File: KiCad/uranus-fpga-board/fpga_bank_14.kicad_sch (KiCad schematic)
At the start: 1 part, among them U12 XC7K325T-3FFG900E

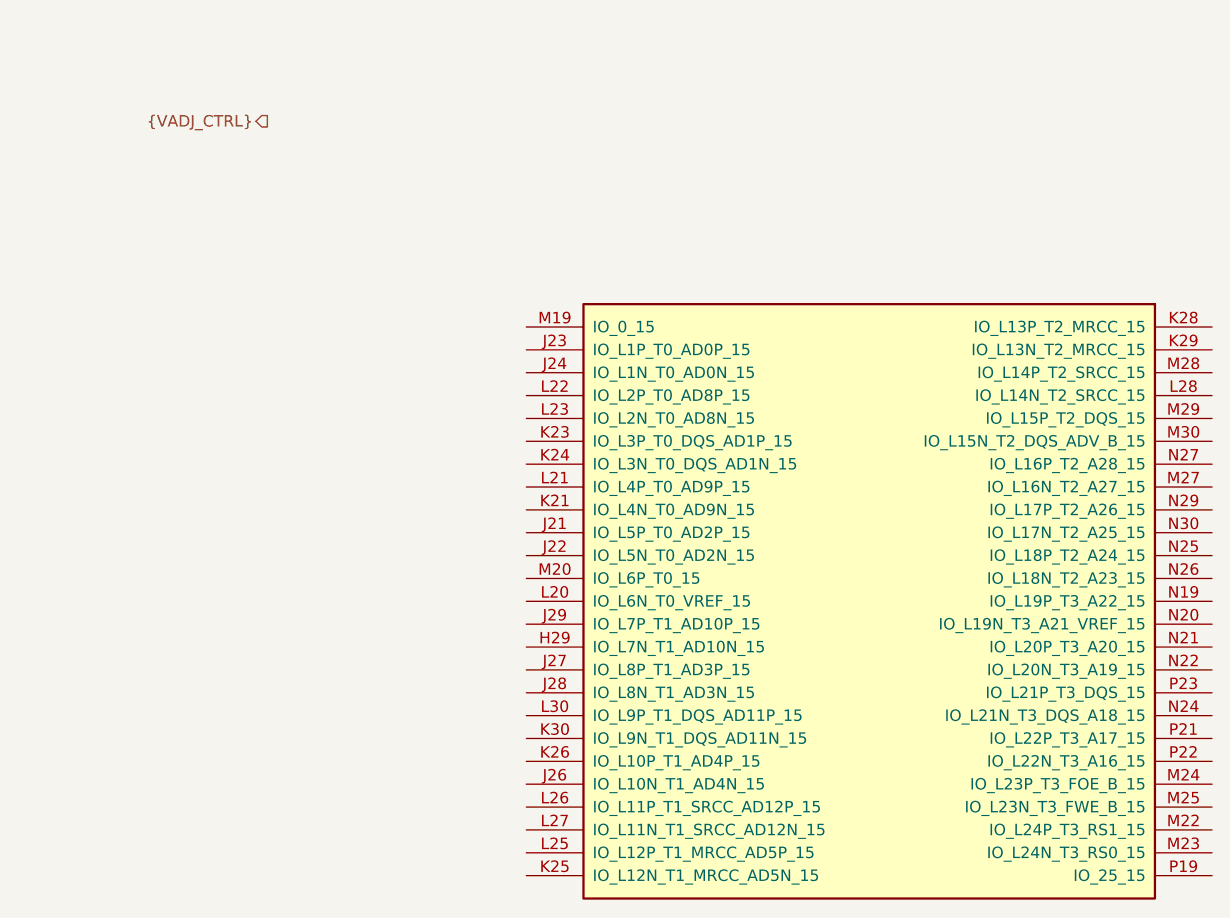
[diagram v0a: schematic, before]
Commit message: I finally did it
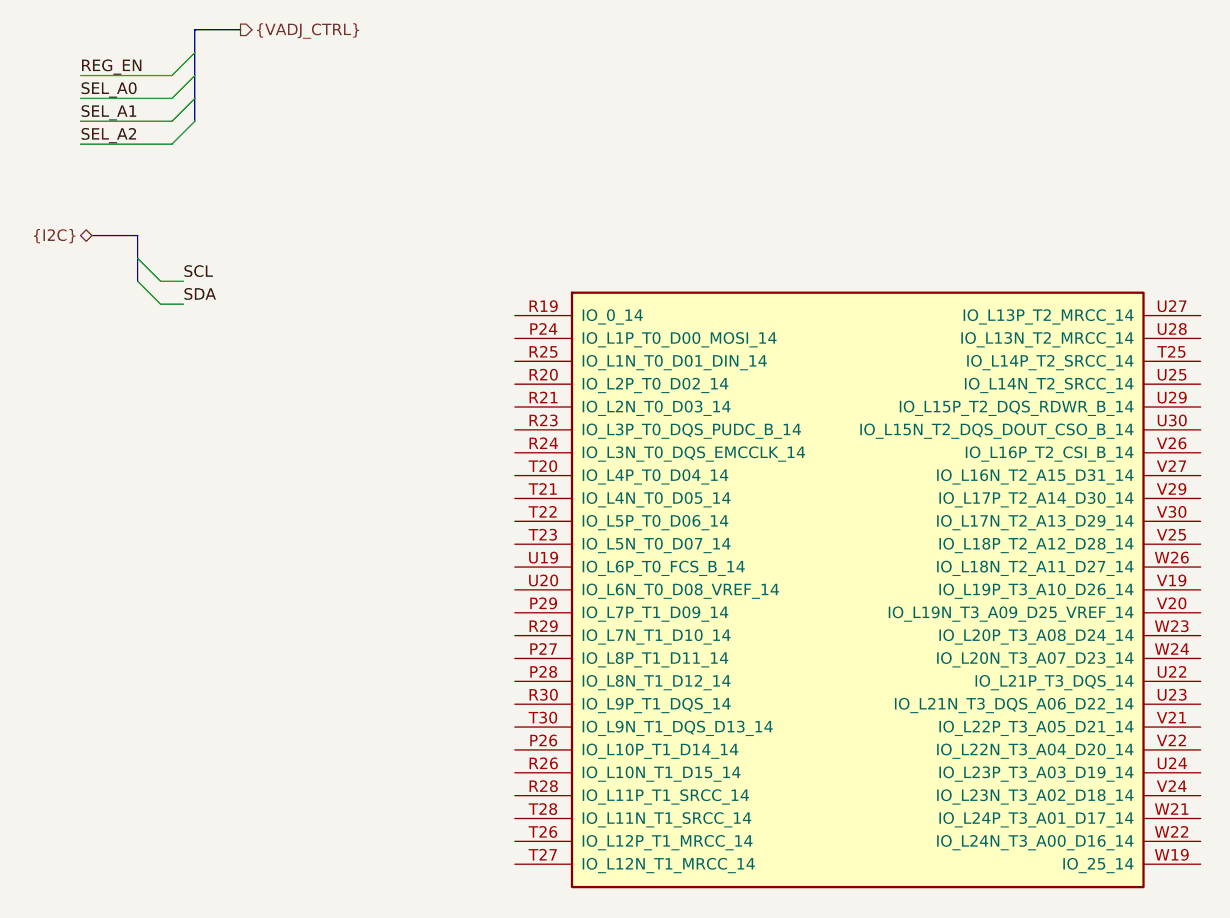
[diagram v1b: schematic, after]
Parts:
- removed U12: XC7K325T-3FFG900E, symbol XC7K325T-3FFG900E:XC7K325T-3FFG900E
- added U1: XC7K325T-3FFG900E, Package_BGA:Xilinx_FFG900_FFG901, symbol XC7K325T-3FFG900E:XC7K325T-3FFG900E
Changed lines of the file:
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@@
 	(generator_version "10.0")
 	(paper "A4")
-	(hierarchical_label "{VADJ_CTRL}"
-		(shape output)
-		(at 77.9155 40.6399 180)
+	(bus_entry
+		(at 69.85 35.56)
+		(size -2.54 2.54)
+		(stroke
+			(width 0)
+			(type default)
+		)
+	)
+	(bus_entry
+		(at 63.5 55.88)
+		(size 2.54 2.54)
+		(stroke
+			(width 0)
+			(type default)
+		)
+	)
+	(bus_entry
+		(at 69.85 38.1)
+		(size -2.54 2.54)
+		(stroke
+			(width 0)
+			(type default)
+		)
+	)
+	(bus_entry
+		(at 63.5 58.42)
+		(size 2.54 2.54)
+		(stroke
+			(width 0)
+			(type default)
+		)
+	)
+	(bus_entry
+		(at 69.85 33.02)
+		(size -2.54 2.54)
+		(stroke
+			(width 0)
+			(type default)
+		)
+	)
+	(bus_entry
+		(at 69.85 40.64)
+		(size -2.54 2.54)
+		(stroke
+			(width 0)
+			(type default)
+		)
+	)
+	(wire
+		(pts
+			(xy 57.15 35.56) (xy 67.31 35.56)
+		)
+		(stroke
+			(width 0)
+			(type default)
+		)
+	)
+	(bus
+		(pts
+			(xy 58.42 53.34) (xy 63.5 53.34)
+		)
+		(stroke
+			(width 0)
+			(type default)
+		)
+	)
+	(wire
+		(pts
+			(xy 57.15 40.64) (xy 67.31 40.64)
+		)
+		(stroke
+			(width 0)
+			(type default)
+		)
+	)
+	(wire
+		(pts
+			(xy 57.15 43.18) (xy 67.31 43.18)
+		)
+		(stroke
+			(width 0)
+			(type default)
+		)
+	)
+	(bus
+		(pts
+			(xy 63.5 53.34) (xy 63.5 58.42)
+		)
+		(stroke
+			(width 0)
+			(type default)
+		)
+	)
+	(wire
+		(pts
+			(xy 66.04 60.96) (xy 68.58 60.96)
+		)
+		(stroke
+			(width 0)
+			(type default)
+		)
+	)
+	(bus
+		(pts
+			(xy 74.93 30.48) (xy 69.85 30.48)
+		)
+		(stroke
+			(width 0)
+			(type default)
+		)
+	)
+	(wire
+		(pts
+			(xy 66.04 58.42) (xy 68.58 58.42)
+		)
+		(stroke
+			(width 0)
+			(type default)
+		)
+	)
+	(bus
+		(pts
+			(xy 69.85 30.48) (xy 69.85 40.64)
+		)
+		(stroke
+			(width 0)
+			(type default)
+		)
+	)
+	(wire
+		(pts
+			(xy 57.15 38.1) (xy 67.31 38.1)
+		)
+		(stroke
+			(width 0)
+			(type default)
+		)
+	)
+	(label "SEL_A2"
+		(at 57.15 43.18 0)
+		(effects
+			(font
+				(size 1.27 1.27)
+			)
+			(justify left bottom)
+		)
+	)
+	(label "SDA"
+		(at 68.58 60.96 0)
+		(effects
+			(font
+				(size 1.27 1.27)
+			)
+			(justify left bottom)
+		)
+	)
+	(label "SEL_A1"
+		(at 57.15 40.64 0)
+		(effects
+			(font
+				(size 1.27 1.27)
+			)
+			(justify left bottom)
+		)
+	)
+	(label "REG_EN"
+		(at 57.15 35.56 0)
+		(effects
+			(font
+				(size 1.27 1.27)
+			)
+			(justify left bottom)
+		)
+	)
+	(label "SEL_A0"
+		(at 57.15 38.1 0)
+		(effects
+			(font
+				(size 1.27 1.27)
+			)
+			(justify left bottom)
+		)
+	)
+	(label "SCL"
+		(at 68.58 58.42 0)
+		(effects
+			(font
+				(size 1.27 1.27)
+			)
+			(justify left bottom)
+		)
+	)
+	(hierarchical_label "{I2C}"
+		(shape bidirectional)
+		(at 58.42 53.34 180)
 		(effects
 			(font
@@
 		)
 	)
+	(hierarchical_label "{VADJ_CTRL}"
+		(shape output)
+		(at 74.93 30.48 0)
+		(effects
+			(font
+				(size 1.27 1.27)
+			)
+			(justify left)
+		)
+	)
 	(symbol
+		(lib_name "XC7K325T-3FFG900E_1")
 		(lib_id "XC7K325T-3FFG900E:XC7K325T-3FFG900E")
-		(at 144.78 93.98 0)
-		(unit 4)
+		(at 143.51 92.71 0)
+		(unit 3)
 		(body_style 1)
 		(exclude_from_sim no)
@@
 		(dnp no)
 		(fields_autoplaced yes)
-		(property "Reference" "U12"
-			(at 144.78 92.71 0)
+		(property "Reference" "U1"
+			(at 143.51 91.44 0)
 			(hide yes)
 			(show_name no)
@@
 		)
 		(property "Value" "XC7K325T-3FFG900E"
-			(at 144.78 95.25 0)
+			(at 143.51 93.98 0)
 			(hide yes)
 			(show_name no)
@@
 			)
 		)
-		(property "Footprint" ""
-			(at 144.78 93.98 0)
+		(property "Footprint" "Package_BGA:Xilinx_FFG900_FFG901"
+			(at 143.51 92.71 0)
 			(hide yes)
 			(show_name no)
@@
 		)
 		(property "Datasheet" ""
-			(at 144.78 93.98 0)
+			(at 143.51 92.71 0)
 			(show_name no)
 			(do_not_autoplace no)
@@
 		)
 		(property "Description" "Kintex 7 T 325 XC7K325T-FFG900"
-			(at 144.78 93.98 0)
+			(at 143.51 92.71 0)
 			(hide yes)
 			(show_name no)
@@
 			(project "uranus-fpga-board"
 				(path "/11d4e4d4-71ba-48aa-ae73-e6b6dc32b11b/ae4670d8-3f7e-4e25-83c4-e414aeb132b8/e70af11b-d02c-4276-ba11-71fb729ac221/df160b42-b095-480e-a002-f23f31e7d2a8"
-					(reference "U12")
-					(unit 4)
+					(reference "U1")
+					(unit 3)
 				)
 			)
